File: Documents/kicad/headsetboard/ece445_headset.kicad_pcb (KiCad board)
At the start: 2 copper layers, 49 parts, among them J1 Screw_Terminal_01x02, J2 Conn_01x05_Female, J3 Conn_ARM_JTAG_SWD_10, J4 PJRAN1X1U04X, Q1 AO4485, Q2 SS8050-G, Q3 SS8050-G, SW1 SW_Push, SW2 SW_Push, U1 TPS62933ODRLR, U2 ESP32-S3-WROOM-1-N16R2

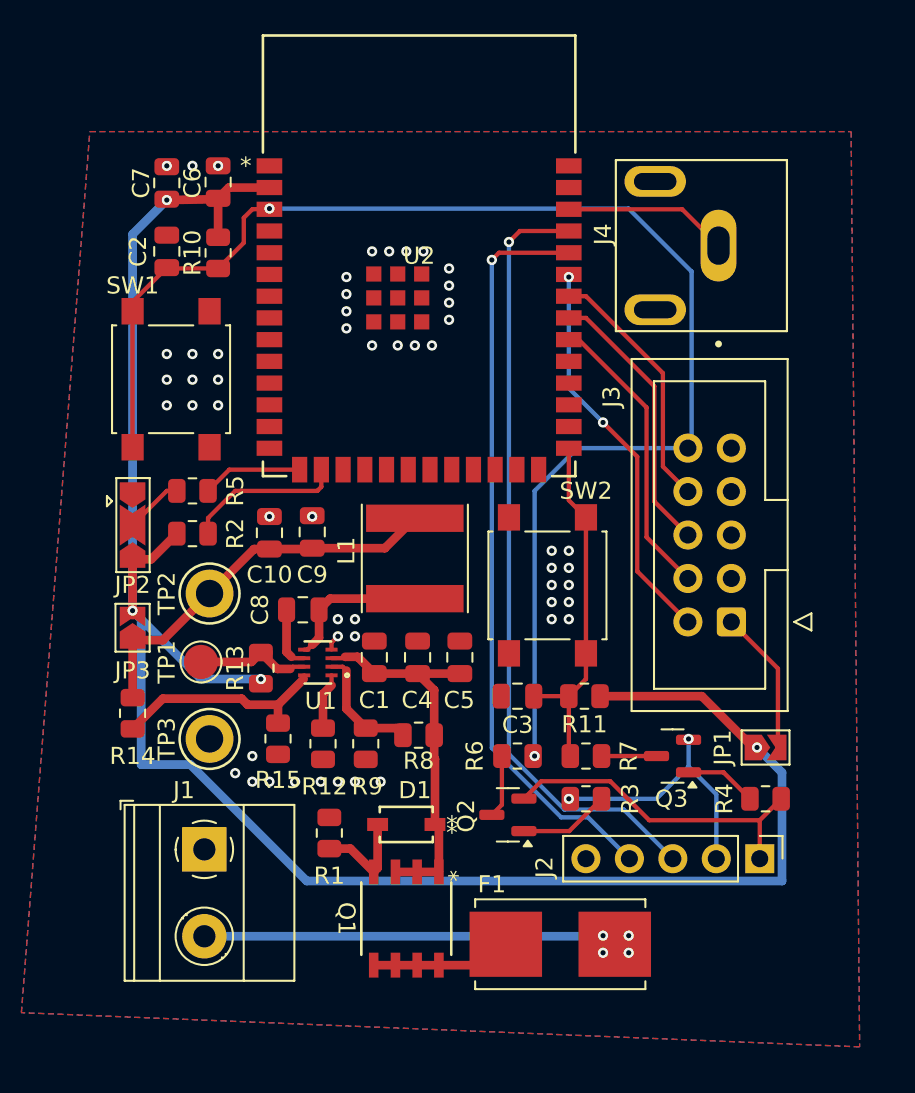
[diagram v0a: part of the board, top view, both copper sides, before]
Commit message: Add files via upload
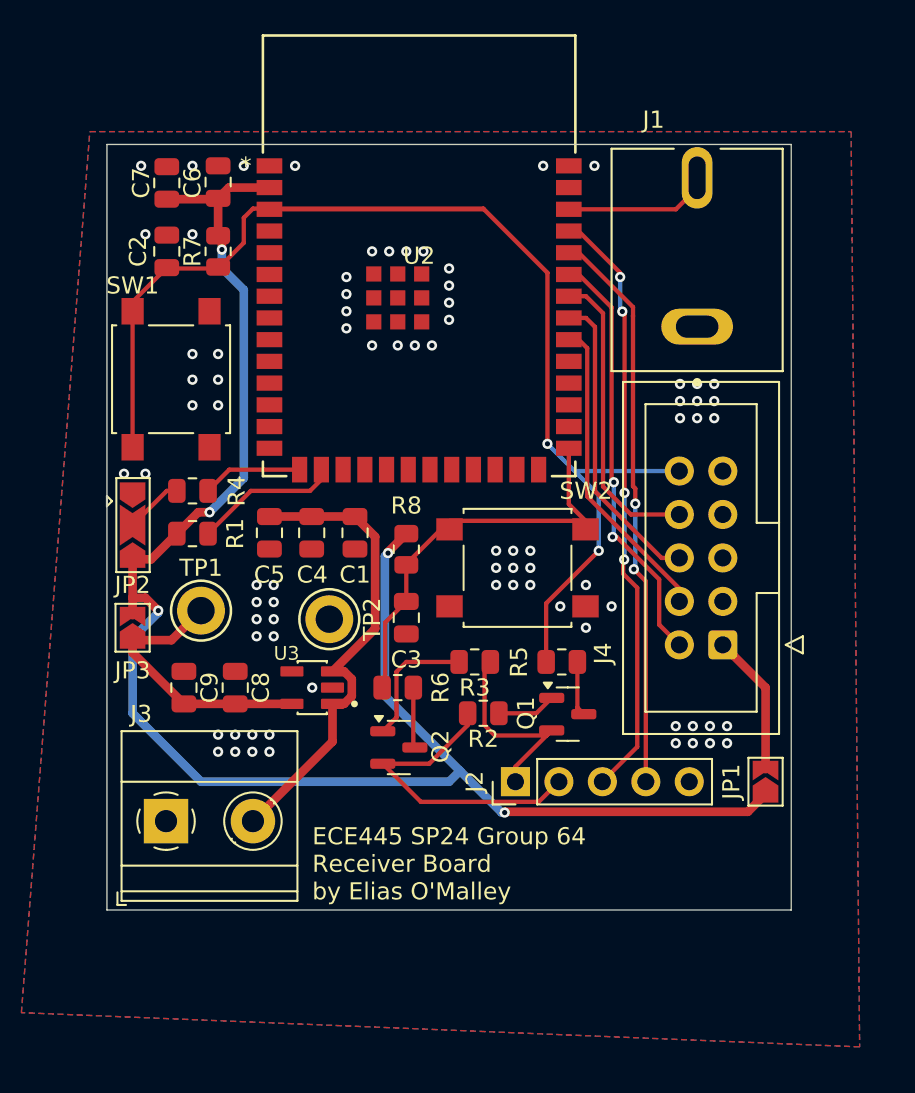
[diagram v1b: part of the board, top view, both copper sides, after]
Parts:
- removed C10: 33u, Capacitor_SMD:C_0805_2012Metric
- removed D1: D_Zener, local_footprints:SOD-123_ONS
- removed F1: Fuse, Fuse:Fuseholder_Littelfuse_Nano2_154x
- removed L1: 4.7u, Inductor_SMD:L_Taiyo-Yuden_NR-60xx
- removed Q3: SS8050-G, Package_TO_SOT_SMD:SOT-23
- removed R10, R11, R13: 100k, Resistor_SMD:R_0805_2012Metric
- removed R12, R9: DNP, Resistor_SMD:R_0805_2012Metric
- removed R14: 31.3k, Resistor_SMD:R_0805_2012Metric
- removed R15: 10.0k, Resistor_SMD:R_0805_2012Metric
- removed TP3: TestPoint, TestPoint:TestPoint_Keystone_5010-5014_Multipurpose
- removed U1: TPS62933ODRLR, local_footprints:SOT5X3-8_DRL_TEX
- added U3: AP2112K-3.3TRG1, csv_conn:SOT95P285X140-5N, F.Cu at (84.5, 78.5)
- C8: value 100n -> 33u
- J1: value Screw_Terminal_01x02 -> RCJ-054; footprint TerminalBlock_Phoenix:TerminalBlock_Phoenix_MKDS-1,5-2-5.08_1x02_P5.08mm_Horizontal -> csv_conn:CUI_RCJ-054
- J3: value Conn_ARM_JTAG_SWD_10 -> Screw_Terminal_01x02; footprint Connector_IDC:IDC-Header_2x05_P2.54mm_Vertical -> TerminalBlock_Phoenix:TerminalBlock_Phoenix_MKDS-1,5-2-5.08_1x02_P5.08mm_Horizontal
- J4: value PJRAN1X1U04X -> Conn_ARM_JTAG_SWD_10; footprint csv_conn:SWITCHCRAFT_PJRAN1X1U04X -> Connector_IDC:IDC-Header_2x05_P2.54mm_Vertical
- Q1: value AO4485 -> SS8050-G; footprint local_footprints:SO8SOP-8L_AOS -> Package_TO_SOT_SMD:SOT-23
- R1: value 100k -> 1k
- R2, R5: value 1k -> 10k
- R4: value 10k -> 1k
- R7: value 10k -> 100k
- R8: value DNP -> 100k
- TP1: footprint TestPoint:TestPoint_Pad_D2.0mm -> TestPoint:TestPoint_Keystone_5010-5014_Multipurpose
- moved J1 46.1 mm to (107.0, 52.0), turned to 0 degrees
- moved R4 38.0 mm to (77.5, 67.0)
- moved R7 36.5 mm to (79.0, 53.0), turned to -90 degrees
- moved J3 35.0 mm to (76.0, 86.3), turned to 0 degrees
- moved R5 23.8 mm to (99.1, 77.0)
- moved J4 23.3 mm to (108.5, 76.0), turned to 180 degrees
- moved R2 20.0 mm to (94.5, 80.0), turned to 0 degrees
- moved R1 19.2 mm to (77.5, 69.5), turned to 180 degrees
- moved Q1 15.2 mm to (99.4, 80.0), turned to 0 degrees
- moved J2 15.0 mm to (96.4, 84.0), turned to 90 degrees
- moved C5 13.3 mm to (82.0, 69.5), turned to -90 degrees
- moved C9 11.8 mm to (77.0, 78.5)
- moved R8 10.9 mm to (90.0, 70.4), turned to -90 degrees
- moved R3 10.3 mm to (94.0, 77.0), turned to 180 degrees
- moved C4 9.56 mm to (84.5, 69.5), turned to -90 degrees
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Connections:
- C8 pad 1: Net-(U1-BST) -> Net-(JP3-A)
- C8 pad 2: Net-(U1-SW) -> GND
- J1 pad 2: Net-(J1-Pin_2) -> /CSV_OUT
- J3 pad 1: Net-(J3-VTref) -> GND
- J3 pad 2: /MTMS -> +BATT
- J4 pad 1: /CSV_OUT -> Net-(J4-VTref)
- J4 pad 2: GND -> /MTMS
- JP1 pad 2: Net-(J3-VTref) -> Net-(J4-VTref)
- Q1 pad 1: +BATT -> Net-(Q1-B)
- Q1 pad 2: +BATT -> /RTS
- Q1 pad 3: +BATT -> Net-(Q1-C)
- Q2 pad 2: /RTS -> /DTR
- R1 pad 1: Net-(D1-A) -> /GPIO46_STRAPPING
- R1 pad 2: GND -> +3V3
- R2 pad 1: /GPIO46_STRAPPING -> /DTR
- R2 pad 2: +3V3 -> Net-(Q1-B)
- R3 pad 1: /DTR -> /RTS
- R4 pad 1: /RTS -> /GPIO3_STRAPPING
- R4 pad 2: Net-(Q3-B) -> Net-(JP2-C)
- R5 pad 1: /GPIO3_STRAPPING -> Net-(Q1-C)
- R5 pad 2: Net-(JP2-C) -> /CHIP_PU
- R6 pad 2: /CHIP_PU -> /GPIO0_STRAPPING
- R7 pad 1: Net-(Q3-C) -> +3V3
- R7 pad 2: /GPIO0_STRAPPING -> /CHIP_PU
- R8 pad 1: +BATT -> +3V3
- R8 pad 2: Net-(U1-EN) -> /GPIO0_STRAPPING
- TP1 pad 1: Net-(U1-PG) -> Net-(JP3-A)
- TP2 pad 1: Net-(JP3-A) -> GND
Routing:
- net Net-(J1-Pin_2): track 32.1 -> 0.00 mm, vias 4 -> 0
- net +3V3: track 118.0 -> 100.0 mm, vias 4 -> 5
- net Net-(U1-FB): track 12.8 -> 0.00 mm
- net /RX: track 43.9 -> 33.8 mm, vias 1 -> 2
- net /TX: track 45.8 -> 35.9 mm, vias 1 -> 4
- net Net-(U1-SW): track 8.67 -> 0.00 mm
- net Net-(J3-VTref): track 8.47 -> 0.00 mm
- net Net-(J4-VTref): track 0.00 -> 8.30 mm
- net Net-(F1-Pad2): track 8.23 -> 0.00 mm
- net Net-(U1-PG): track 7.16 -> 0.00 mm
- net /RTS: track 19.2 -> 12.0 mm
- net Net-(U1-EN): track 7.14 -> 0.00 mm
- net Net-(JP3-A): track 22.8 -> 16.0 mm
- net Net-(D1-A): track 6.03 -> 0.00 mm
- net +BATT: track 22.6 -> 28.1 mm
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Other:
- board outline added: 40 x 44.8 mm
- board text added: "ECE445 SP24 Group 64 Receiver Board by Elias O'Malley"
